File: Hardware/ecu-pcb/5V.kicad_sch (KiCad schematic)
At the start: 20 parts, among them U5 TPS5430DDAR

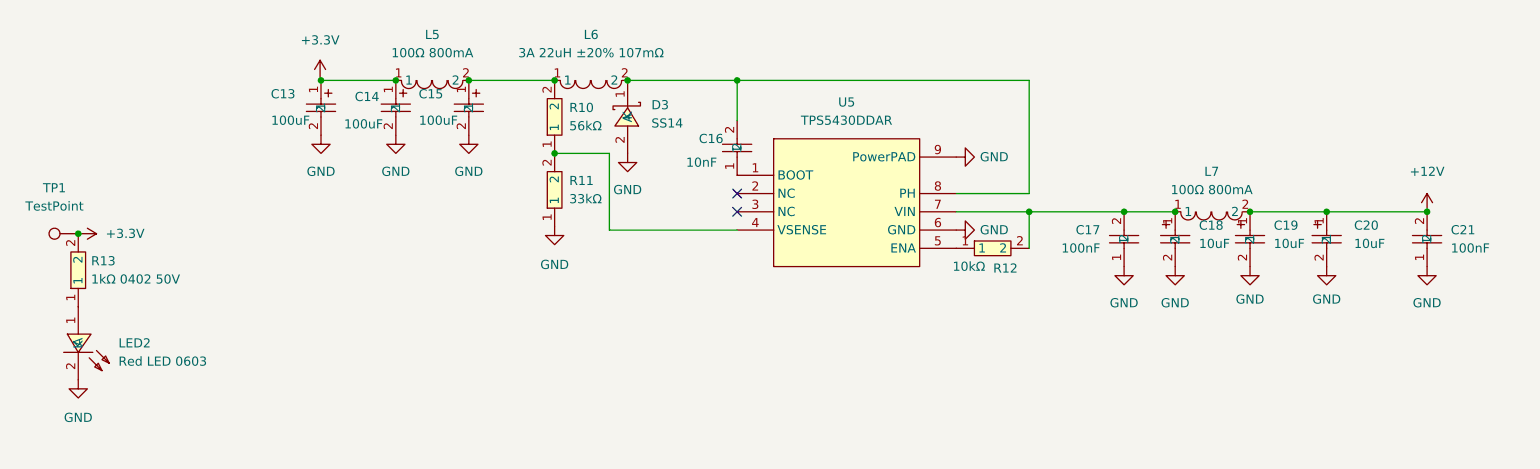
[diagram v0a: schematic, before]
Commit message: Ecu SCH Ready
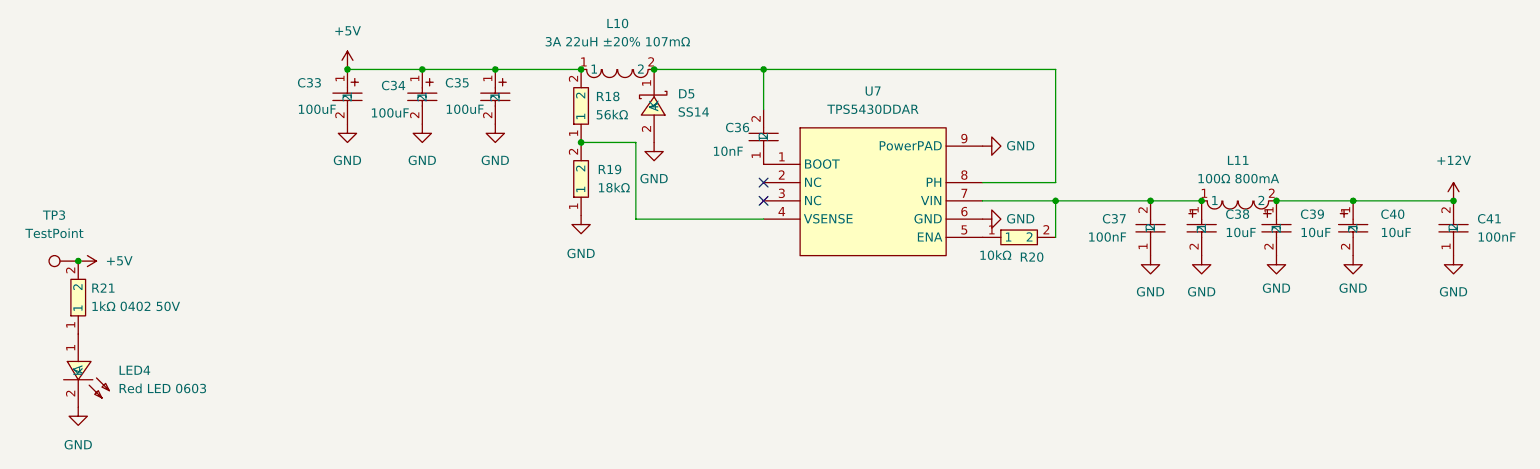
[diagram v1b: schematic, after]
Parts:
- removed C13, C14, C15: 100uF, easyeda2kicad:CAP-SMD_L3.5-W2.8, symbol easyeda2kicad:100uF 6.3V Tantal 3528
- removed C16: 10nF, easyeda2kicad:C0402, symbol easyeda2kicad:50V 10nF X7R ±10% 0402
- removed C17, C21: 100nF, easyeda2kicad:C0402_NEW, symbol easyeda2kicad:16V 100nF X7R ±10% 0402
- removed C18, C19, C20: 10uF, easyeda2kicad:CAP-SMD_L3.2-W1.6-RD-C7171, symbol easyeda2kicad:10uF 16V Tantal 3216
- removed D3: SS14, easyeda2kicad:SMA_L4.2-W2.6-LS5.3-RD, symbol easyeda2kicad:SS14
- removed L5, L7: 100Ω 800mA, easyeda2kicad:L0805, symbol easyeda2kicad:100Ω 800mA
- removed L6: 3A 22uH ±20% 107mΩ, easyeda2kicad:IND-SMD_L7.3-W6.6, symbol easyeda2kicad: 3A 22uH ±20% 107mΩ
- removed LED2: Red LED 0603, easyeda2kicad:LED0603-R-RD, symbol easyeda2kicad:Red LED 0603
- removed R10: 56kΩ, easyeda2kicad:R0402, symbol easyeda2kicad:56kΩ 0402 50V
- removed R11: 33kΩ, easyeda2kicad:R0402, symbol easyeda2kicad:33kΩ 0402 50V
- removed R12: 10kΩ, easyeda2kicad:R0402, symbol easyeda2kicad:10kΩ 0402 50V
- removed R13: 1kΩ 0402 50V, easyeda2kicad:R0402, symbol easyeda2kicad:1kΩ 0402 50V
- removed TP1: TestPoint, TestPoint:TestPoint_Loop_D2.50mm_Drill1.0mm_LowProfile, symbol Connector:TestPoint
- removed U5: TPS5430DDAR, easyeda2kicad:ESOP-8_L4.9-W3.9-P1.27-LS6.0-TL-EP, symbol easyeda2kicad:TPS5430DDAR
- added C33, C34, C35: 100uF, easyeda2kicad:CAP-SMD_L3.5-W2.8, symbol easyeda2kicad:100uF 6.3V Tantal 3528
- added C36: 10nF, easyeda2kicad:C0402, symbol easyeda2kicad:50V 10nF X7R ±10% 0402
- added C37, C41: 100nF, easyeda2kicad:C0402_NEW, symbol easyeda2kicad:16V 100nF X7R ±10% 0402
- added C38, C39, C40: 10uF, easyeda2kicad:CAP-SMD_L3.2-W1.6-RD-C7171, symbol easyeda2kicad:10uF 16V Tantal 3216
- added D5: SS14, easyeda2kicad:SMA_L4.2-W2.6-LS5.3-RD, symbol easyeda2kicad:SS14
- added L10: 3A 22uH ±20% 107mΩ, easyeda2kicad:IND-SMD_L7.3-W6.6, symbol easyeda2kicad: 3A 22uH ±20% 107mΩ
- added L11: 100Ω 800mA, easyeda2kicad:L0805, symbol easyeda2kicad:100Ω 800mA
- added LED4: Red LED 0603, easyeda2kicad:LED0603-R-RD, symbol easyeda2kicad:Red LED 0603
- added R18: 56kΩ, easyeda2kicad:R0402, symbol easyeda2kicad:56kΩ 0402 50V
- added R19: 18kΩ, easyeda2kicad:R0402, symbol easyeda2kicad:18kΩ 0402 50V
- added R20: 10kΩ, easyeda2kicad:R0402, symbol easyeda2kicad:10kΩ 0402 50V
- added R21: 1kΩ 0402 50V, easyeda2kicad:R0402, symbol easyeda2kicad:1kΩ 0402 50V
- added TP3: TestPoint, symbol Connector:TestPoint
- added U7: TPS5430DDAR, easyeda2kicad:ESOP-8_L4.9-W3.9-P1.27-LS6.0-TL-EP, symbol easyeda2kicad:TPS5430DDAR
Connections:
- net +12V: now also C39.1, C40.1, C41.2, L11.2
- net GND: now also C33.2, C34.2, C35.2, C37.1, C38.2, C39.2, C40.2, C41.1, D5.2 (A), LED4.2 (K), R19.1, U7.6 (GND), U7.9 (PowerPAD)
- new net: C36.2, D5.1 (K), L10.2, U7.8 (PH)
- new net: C36.1, U7.1 (BOOT)
- new net: R18.1, R19.2, U7.4 (VSENSE)
- new net: R20.1, U7.5 (ENA)
- new net: C37.2, C38.1, L11.1, R20.2, U7.7 (VIN)
- new net: LED4.1 (A), R21.1
- new net +5V: C33.1, C34.1, C35.1, L10.1, R18.2, R21.2, TP3.1

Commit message: Updated Schematic
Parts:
- TP3: footprint (none) -> TestPoint:TestPoint_Loop_D2.50mm_Drill1.0mm_LowProfile
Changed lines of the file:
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@@
     (property "Reference" "TP3" (id 0) (at 28.448 87.63 90))
     (property "Value" "TestPoint" (id 1) (at 28.448 90.17 90))
-    (property "Footprint" "" (id 2) (at 31.75 88.9 0)
+    (property "Footprint" "TestPoint:TestPoint_Loop_D2.50mm_Drill1.0mm_LowProfile" (id 2) (at 31.75 88.9 0)
       (effects (font (size 1.27 1.27)) hide)
     )
